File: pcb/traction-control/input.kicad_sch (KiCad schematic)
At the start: 16 parts, among them Q7 AO3401A, Q8 AO3400A, Q9 AO3400A, U5 LM393

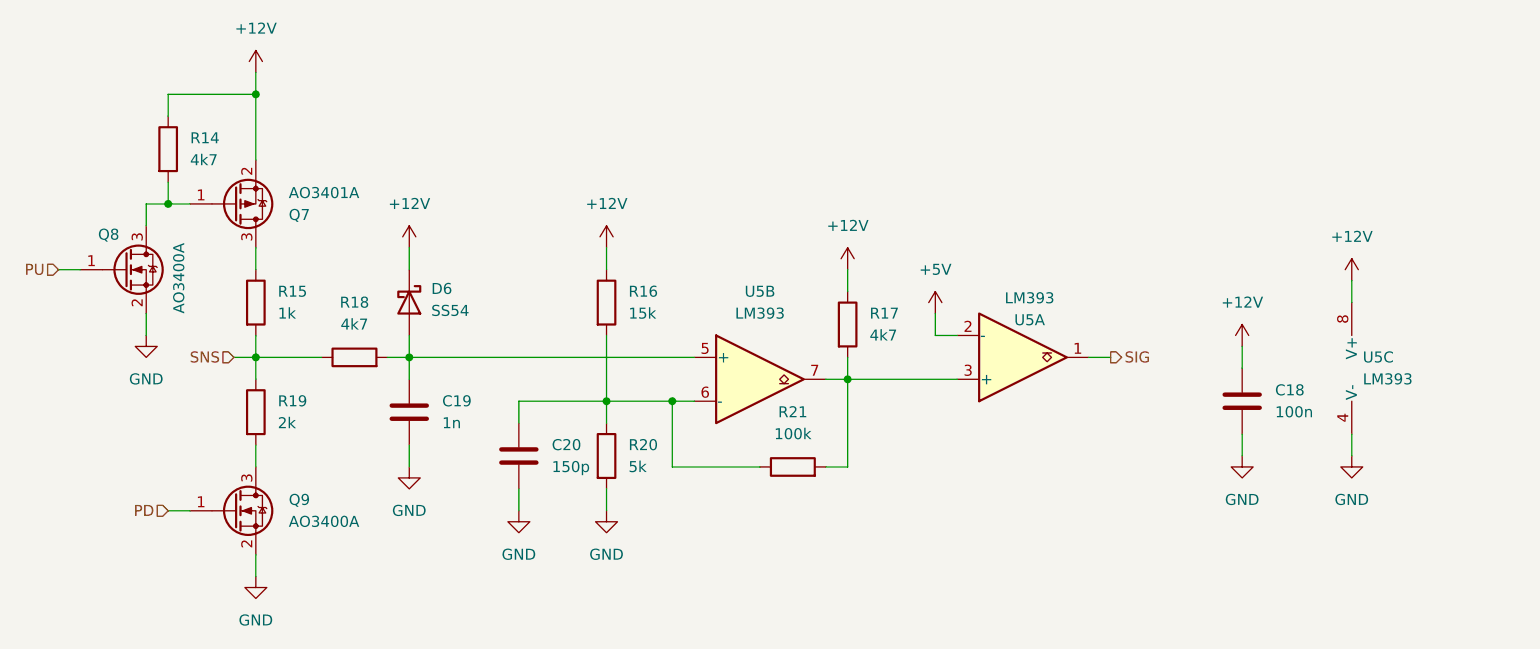
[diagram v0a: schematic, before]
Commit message: Revision and production files
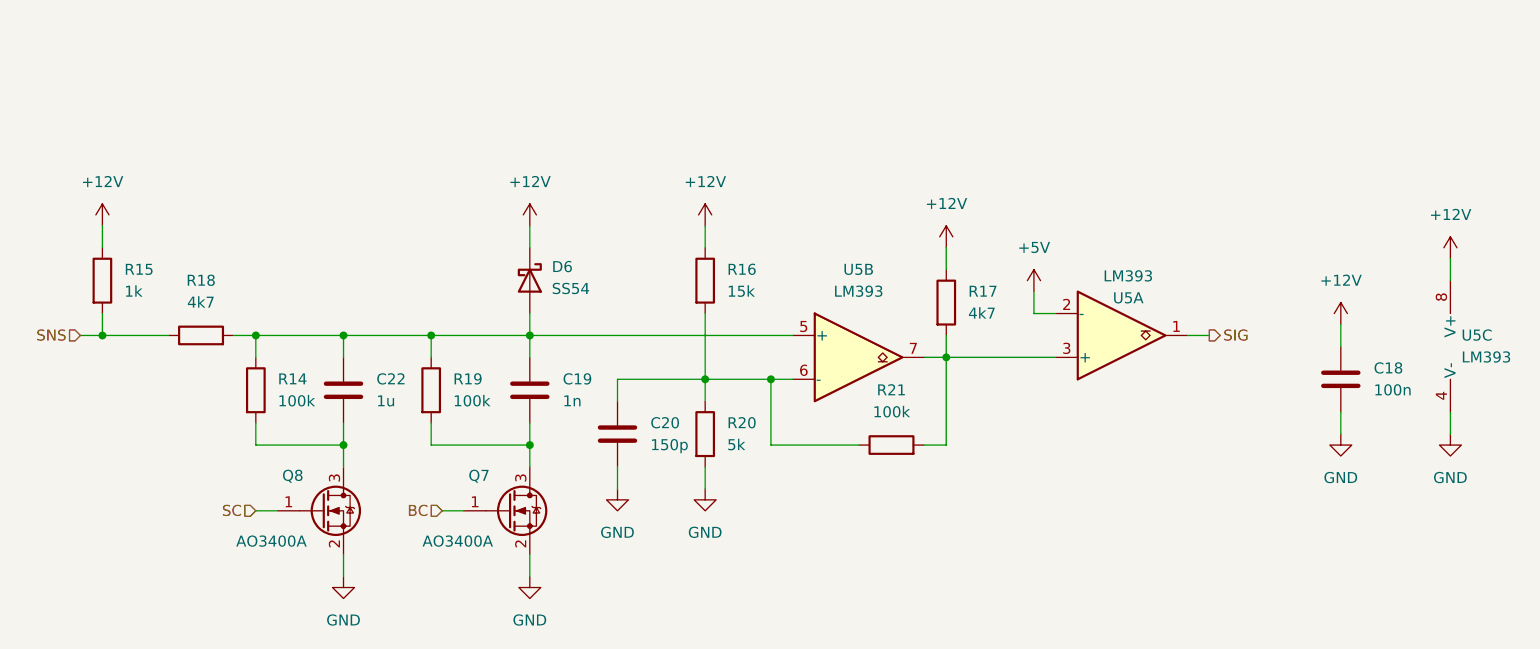
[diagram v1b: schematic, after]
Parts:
- removed Q7: AO3401A, Package_TO_SOT_SMD:SOT-23, symbol Transistor_FET:AO3401A
- removed Q9: AO3400A, Package_TO_SOT_SMD:SOT-23, symbol Transistor_FET:AO3400A
- added C22: 1u, Capacitor_SMD:C_0402_1005Metric, symbol Device:C
- added Q7: AO3400A, Package_TO_SOT_SMD:SOT-23, symbol Transistor_FET:AO3400A
- R14: value 4k7 -> 100k
- R19: value 2k -> 100k; footprint Resistor_SMD:R_1206_3216Metric -> Resistor_SMD:R_0402_1005Metric
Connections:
- net +12V: now also R15.1; no longer R14.1
- net GND: now also Q7.2 (S); no longer C19.2
- net SNS: no longer R19.1
- net at Q8.3 (D), R14.2: now also C22.2
- net at C19.1, D6.2 (A), R18.2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: now also R14.1, R19.1, C22.1
- net at R19.2: now also C19.2, Q7.3 (D)
- net PU renamed SC
- new net BC: Q7.1 (G)
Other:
- moved on the sheet: C18, C19, C20, D6, R15, R16, R17, R18, R20, R21, U5A, U5B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
